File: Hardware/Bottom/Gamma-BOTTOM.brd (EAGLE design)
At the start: 33 x 33 mm, 32 parts, among them U1 AD5242-SO16

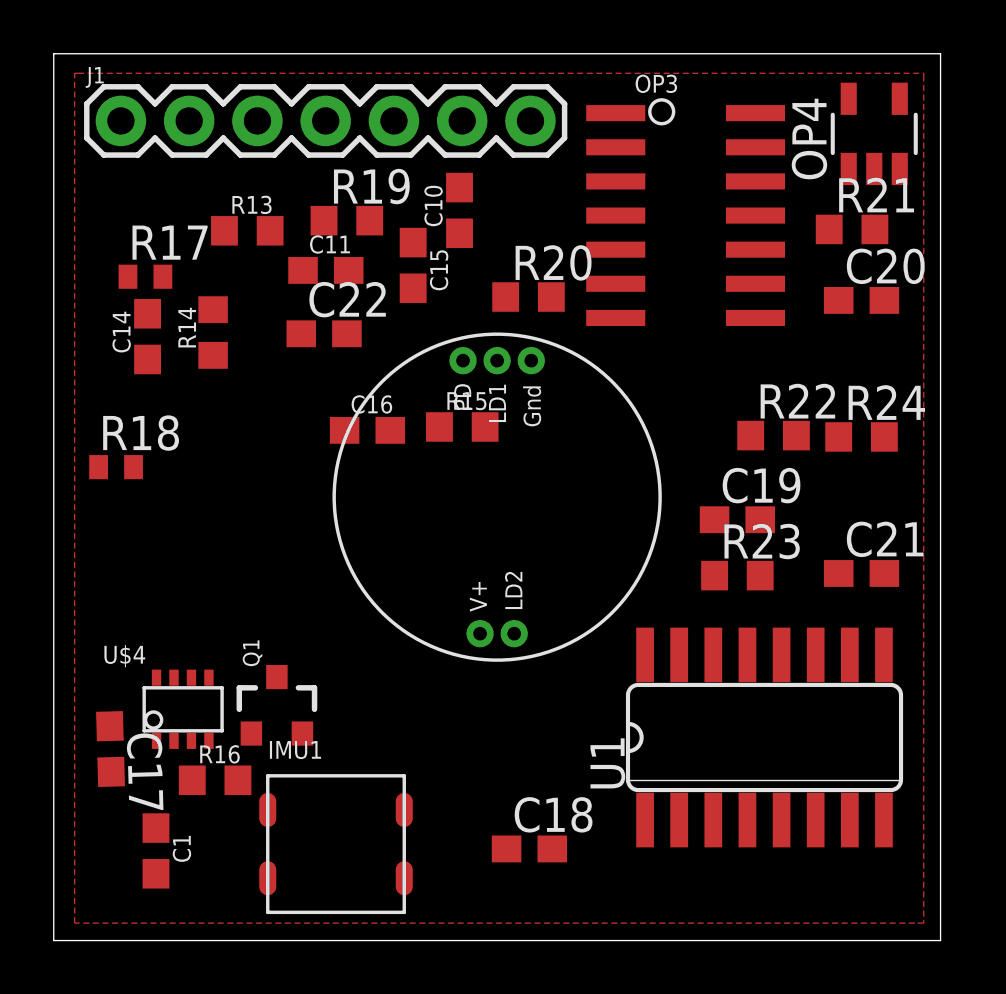
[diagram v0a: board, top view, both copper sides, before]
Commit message: Finished Bottom Board as of Take 003
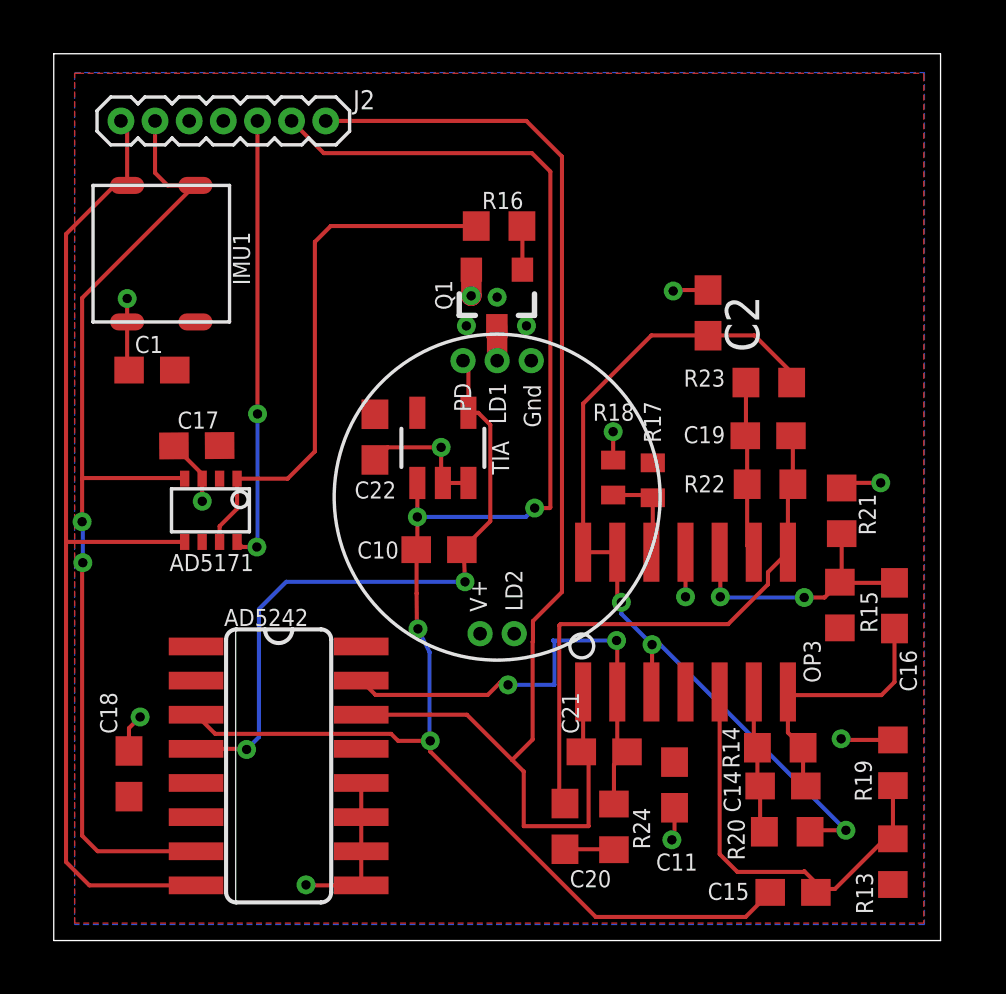
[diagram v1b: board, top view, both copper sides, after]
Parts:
- removed J1: (no value), LinnesLab-Connectors:1X07
- removed OP4: (no value), LinnesLab-AnalogIC:SOT23-5
- removed U$4: AD5171, LinnesLab-DigitalIC:SOT-23-8
- removed U1: AD5242-SO16, LinnesLab-DigitalIC:SO16
- added AD5171: AD5171, LinnesLab-DigitalIC:SOT-23-8
- added AD5242: AD5242-SO16, LinnesLab-DigitalIC:SO16
- added C2: 100n, LinnesLab-Passives:C0603
- added J2: (no value), LinnesLab-Connectors:1X07_1.27MM
- added TIA: (no value), LinnesLab-AnalogIC:SOT23-5
- moved R13 33.6 mm to (33.7, 5.44), turned to 270 degrees
- moved C14 29.0 mm to (29.6, 8.25), turned to 180 degrees
- moved R19 28.6 mm to (33.7, 9.12), turned to 270 degrees
- moved C15 27.3 mm to (30.0, 4.29), turned to 0 degrees
- moved R14 26.2 mm to (29.5, 9.67), turned to 0 degrees
- moved R16 23.2 mm to (19.1, 29.1)
- moved C11 23.1 mm to (25.6, 8.29), turned to 90 degrees
- moved IMU1 22.9 mm to (6.50, 28.1), turned to 90 degrees
- moved C20 22.5 mm to (21.5, 6.75), turned to 270 degrees
- moved R20 22.1 mm to (29.8, 6.55), turned to 180 degrees
- moved C16 20.7 mm to (33.8, 15.0), turned to 90 degrees
- moved R17 20.3 mm to (24.8, 19.6), turned to 90 degrees
- moved R18 18.5 mm to (23.3, 19.7), turned to 270 degrees
- moved C1 17.9 mm to (6.15, 23.7), turned to 0 degrees
- moved Q1 17.3 mm to (19.0, 26.5), turned to 180 degrees
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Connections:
- removed net LED: Q1.3
- net 3.3V: now also AD5171.2, AD5171.6, AD5242.5, AD5242.6, J2.4, TIA.5; no longer OP4.5, U$4.2, U$4.6, U1.5, U1.6
- net A6/TIA: now also AD5242.3, J2.6, TIA.1; no longer J1.5, OP4.1, U1.3
- net A7/PPG: now also AD5242.14, J2.7; no longer J1.7, U1.14
- net D29/LED.CTRL: now also AD5171.8, J2.5; no longer J1.6, U$4.8
- net G.A1: now also AD5242.2; no longer U1.2
- net G.A2: now also AD5242.16; no longer U1.16
- net G.O1: now also AD5242.1; no longer U1.1
- net G.O2: now also AD5242.13; no longer U1.13
- net G.W2: now also AD5242.15; no longer U1.15
- net GND: now also AD5171.3, AD5242.10, AD5242.11, AD5242.12, AD5242.9, C2.1, J2.3, TIA.2, TIA.3; no longer OP4.2, OP4.3, U$4.3, U1.10, U1.11, U1.12, U1.9
- net LED.C: now also Q1.3
- net N$9: now also AD5171.1, AD5171.7; no longer U$4.1, U$4.7
- net PD.C: now also AD5242.4, TIA.4; no longer OP4.4, U1.4
- net SCL: now also AD5171.4, AD5242.7, J2.2; no longer U$4.4, U1.7
- net SDA: now also AD5171.5, AD5242.8, J2.1; no longer U$4.5, U1.8
- net VREF: now also C2.2
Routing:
- net A6/TIA: track 0.00 -> 62.9 mm, vias 0 -> 4
- net A7/PPG: track 0.00 -> 49.1 mm
- net SDA: track 0.00 -> 38.7 mm
- net SCL: track 0.00 -> 37.9 mm, vias 0 -> 2
- net VREF: track 0.00 -> 33.7 mm, vias 0 -> 3
- net GND: track 0.00 -> 27.2 mm, vias 0 -> 15
- net PD.C: track 0.00 -> 24.7 mm, vias 0 -> 2
- net N$19: track 0.00 -> 21.1 mm
- net N$9: track 0.00 -> 20.0 mm
- net G.W2: track 0.00 -> 18.1 mm, vias 0 -> 2
- net D29/LED.CTRL: track 0.00 -> 16.7 mm, vias 0 -> 2
- net N$13: track 0.00 -> 16.1 mm
- net N$17: track 0.00 -> 10.2 mm, vias 0 -> 2
- net N$16: track 0.00 -> 9.94 mm
- net N$18: track 0.00 -> 6.45 mm
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- added copper zone on layer 16, net GND
